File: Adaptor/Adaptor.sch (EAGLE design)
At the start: 10 parts

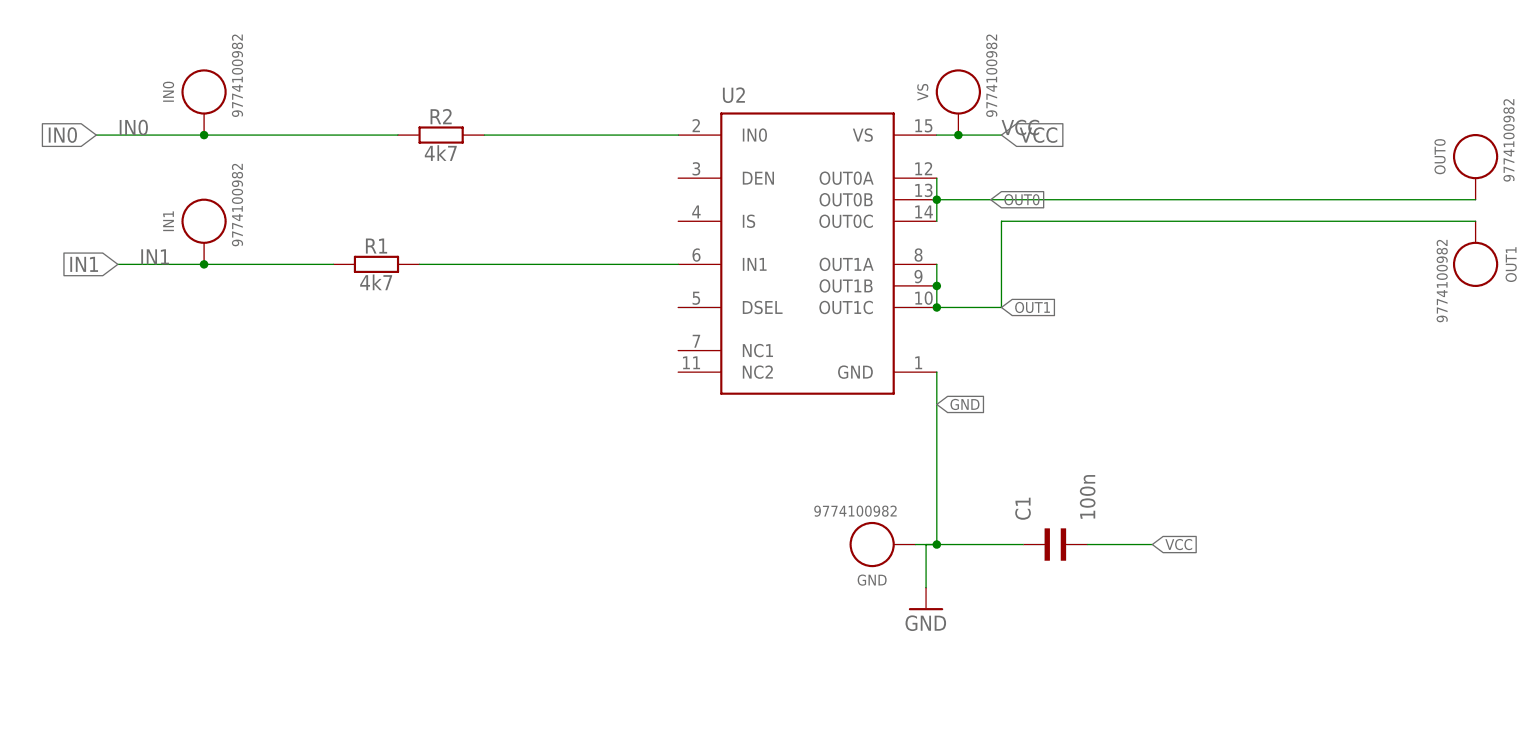
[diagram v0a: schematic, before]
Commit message: cleanm up.
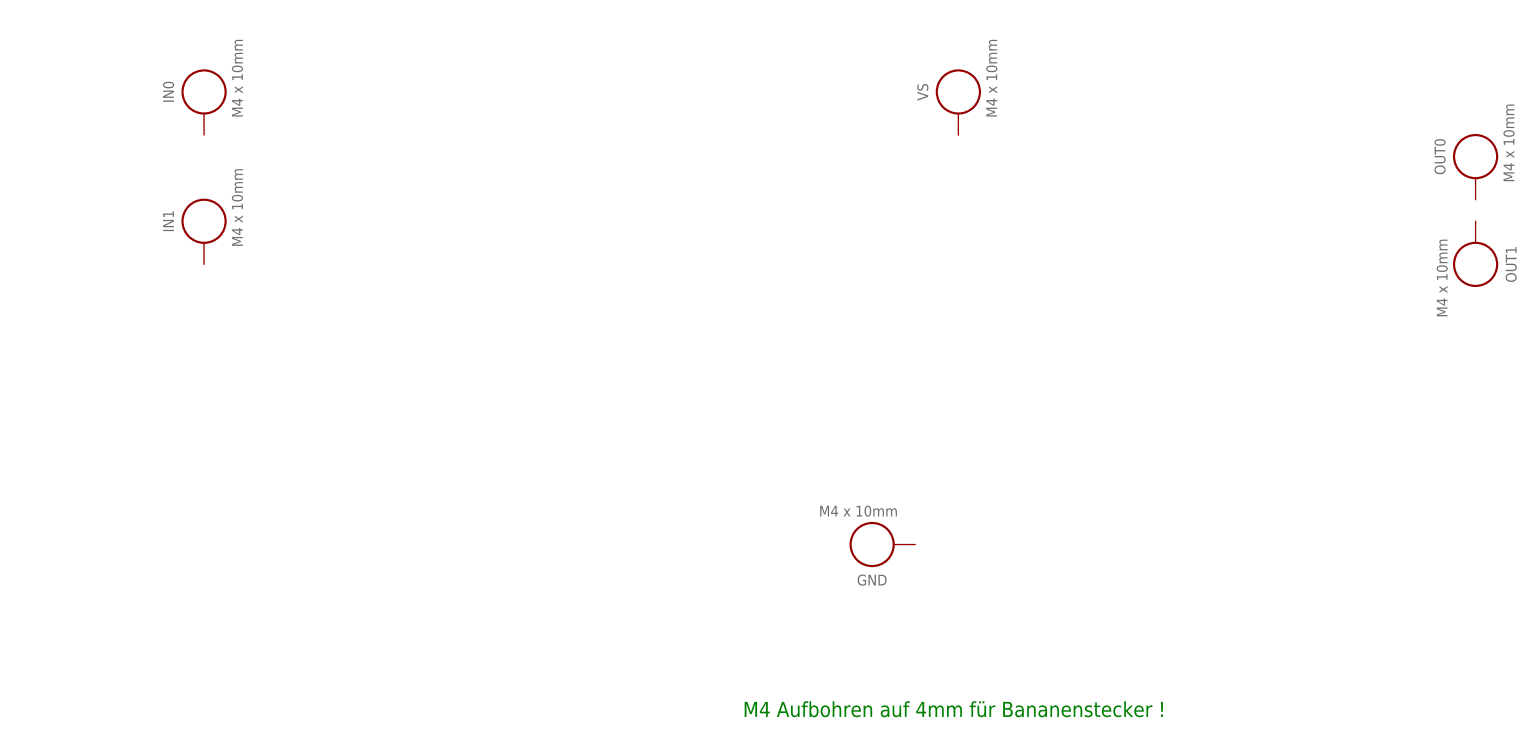
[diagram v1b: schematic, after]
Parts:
- removed C1: 100n, Wurth_Elektronik_Passive_Capacitors_rev19a:WCAP-CSGP_0402_885012205037
- removed R1, R2: 4k7, Resistor_smaller_fliegl:R-EU_WCAP-CSGP_0402
- removed U2: (no value), BTS7030-2EPA:BTS7030-2EPA
- GND, IN0, IN1, OUT0, OUT1, VS: value 9774100982 -> M4 x 10mm; device Wurth_Assembly_WA-SMST:WA-SMST_9774XXX982_9774100982 -> Wurth_Assembly_WA-SMSI:WA-SMSI_9774XXX482_9774100482
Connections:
- removed net GND: C1.2, GND.1, U2.GND
- removed net IN0: IN0.1, R2.1
- removed net IN1: IN1.1, R1.1
- removed net N$16: R2.2, U2.IN0
- removed net N$18: R1.2, U2.IN1
- removed net OUT0: OUT0.1, U2.OUT0A, U2.OUT0B, U2.OUT0C
- removed net OUT1: OUT1.1, U2.OUT1A, U2.OUT1B, U2.OUT1C
- removed net VCC: C1.1, U2.VS, VS.1
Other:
- note added: "M4 Aufbohren auf 4mm für Bananenstecker !"
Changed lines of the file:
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@@
 <drawing>
 <settings>
-<setting alwaysvectorfont="yes"/>
+<setting alwaysvectorfont="no"/>
 <setting verticaltext="up"/>
 </settings>
@@
 </classes>
 <parts>
-<part name="U2" library="BTS7030-2EPA" deviceset="BTS7030-2EPA" device=""/>
-<part name="R2" library="Resistor_smaller_fliegl" deviceset="R-EU_" device="WCAP-CSGP_0402" package3d_urn="urn:adsk.eagle:package:18563160/2" value="4k7"/>
-<part name="R1" library="Resistor_smaller_fliegl" deviceset="R-EU_" device="WCAP-CSGP_0402" package3d_urn="urn:adsk.eagle:package:18563160/2" value="4k7"/>
-<part name="GND21" library="supply1" library_urn="urn:adsk.eagle:library:371" deviceset="GND" device=""/>
-<part name="C1" library="Wurth_Elektronik_Passive_Capacitors_rev19a" library_urn="urn:adsk.eagle:library:491551" deviceset="WCAP-CSGP_0402" device="" package3d_urn="urn:adsk.eagle:package:491821/3" technology="_885012205037" value="100n"/>
-<part name="IN0" library="Wurth_Assembly_WA-SMST" library_urn="urn:adsk.eagle:library:14418621" deviceset="WA-SMST_9774XXX982" device="_9774100982" package3d_urn="urn:adsk.eagle:package:14328907/2" value=" 9774100982 "/>
-<part name="IN1" library="Wurth_Assembly_WA-SMST" library_urn="urn:adsk.eagle:library:14418621" deviceset="WA-SMST_9774XXX982" device="_9774100982" package3d_urn="urn:adsk.eagle:package:14328907/2" value=" 9774100982 "/>
-<part name="GND" library="Wurth_Assembly_WA-SMST" library_urn="urn:adsk.eagle:library:14418621" deviceset="WA-SMST_9774XXX982" device="_9774100982" package3d_urn="urn:adsk.eagle:package:14328907/2" value=" 9774100982 "/>
-<part name="OUT1" library="Wurth_Assembly_WA-SMST" library_urn="urn:adsk.eagle:library:14418621" deviceset="WA-SMST_9774XXX982" device="_9774100982" package3d_urn="urn:adsk.eagle:package:14328907/2" value=" 9774100982 "/>
-<part name="OUT0" library="Wurth_Assembly_WA-SMST" library_urn="urn:adsk.eagle:library:14418621" deviceset="WA-SMST_9774XXX982" device="_9774100982" package3d_urn="urn:adsk.eagle:package:14328907/2" value=" 9774100982 "/>
-<part name="VS" library="Wurth_Assembly_WA-SMST" library_urn="urn:adsk.eagle:library:14418621" deviceset="WA-SMST_9774XXX982" device="_9774100982" package3d_urn="urn:adsk.eagle:package:14328907/2" value=" 9774100982 "/>
+<part name="IN0" library="Wurth_Assembly_WA-SMSI" library_urn="urn:adsk.eagle:library:14418591" deviceset="WA-SMSI_9774XXX482" device="_9774100482" package3d_urn="urn:adsk.eagle:package:14321898/2" value="M4 x 10mm"/>
+<part name="IN1" library="Wurth_Assembly_WA-SMSI" library_urn="urn:adsk.eagle:library:14418591" deviceset="WA-SMSI_9774XXX482" device="_9774100482" package3d_urn="urn:adsk.eagle:package:14321898/2" value="M4 x 10mm"/>
+<part name="GND" library="Wurth_Assembly_WA-SMSI" library_urn="urn:adsk.eagle:library:14418591" deviceset="WA-SMSI_9774XXX482" device="_9774100482" package3d_urn="urn:adsk.eagle:package:14321898/2" value="M4 x 10mm"/>
+<part name="OUT1" library="Wurth_Assembly_WA-SMSI" library_urn="urn:adsk.eagle:library:14418591" deviceset="WA-SMSI_9774XXX482" device="_9774100482" package3d_urn="urn:adsk.eagle:package:14321898/2" value="M4 x 10mm"/>
+<part name="OUT0" library="Wurth_Assembly_WA-SMSI" library_urn="urn:adsk.eagle:library:14418591" deviceset="WA-SMSI_9774XXX482" device="_9774100482" package3d_urn="urn:adsk.eagle:package:14321898/2" value="M4 x 10mm"/>
+<part name="VS" library="Wurth_Assembly_WA-SMSI" library_urn="urn:adsk.eagle:library:14418591" deviceset="WA-SMSI_9774XXX482" device="_9774100482" package3d_urn="urn:adsk.eagle:package:14321898/2" value="M4 x 10mm"/>
 </parts>
 <sheets>
 <sheet>
 <plain>
+<text x="86.36" y="5.08" size="1.778" layer="91">M4 Aufbohren auf 4mm für Bananenstecker !</text>
 </plain>
 <instances>
-<instance part="U2" gate="G$1" x="83.82" y="76.2" smashed="yes">
-<attribute name="NAME" x="83.82" y="77.47" size="1.778" layer="95"/>
-<attribute name="VALUE" x="83.82" y="40.005" size="1.778" layer="96"/>
-</instance>
-<instance part="R2" gate="G$1" x="50.8" y="73.66" smashed="yes">
-<attribute name="NAME" x="50.8" y="74.93" size="1.778" layer="95" align="bottom-center"/>
-<attribute name="VALUE" x="50.8" y="72.39" size="1.778" layer="96" align="top-center"/>
-</instance>
-<instance part="R1" gate="G$1" x="43.18" y="58.42" smashed="yes">
-<attribute name="NAME" x="43.18" y="59.69" size="1.778" layer="95" align="bottom-center"/>
-<attribute name="VALUE" x="43.18" y="57.15" size="1.778" layer="96" align="top-center"/>
-</instance>
-<instance part="GND21" gate="1" x="107.95" y="17.78" smashed="yes">
-<attribute name="VALUE" x="105.41" y="15.24" size="1.778" layer="96"/>
-</instance>
-<instance part="C1" gate="G$1" x="124.46" y="25.4" smashed="yes" rot="R90">
-<attribute name="NAME" x="120.269" y="28.194" size="1.778" layer="95" rot="R90"/>
-<attribute name="VALUE" x="127.889" y="28.194" size="1.778" layer="96" rot="R90"/>
-</instance>
 <instance part="IN0" gate="G$1" x="22.86" y="78.74" smashed="yes" rot="R90">
 <attribute name="NAME" x="19.304" y="78.74" size="1.27" layer="95" rot="R90" align="bottom-center"/>
@@
 </busses>
 <nets>
-<net name="GND" class="0">
-<segment>
-<pinref part="GND21" gate="1" pin="GND"/>
-<wire x1="107.95" y1="25.4" x2="107.95" y2="20.32" width="0.1524" layer="91"/>
-<wire x1="107.95" y1="25.4" x2="109.22" y2="25.4" width="0.1524" layer="91"/>
-<pinref part="C1" gate="G$1" pin="2"/>
-<pinref part="U2" gate="G$1" pin="GND"/>
-<label x="109.22" y="41.91" size="1.27" layer="95" xref="yes"/>
-<wire x1="109.22" y1="25.4" x2="119.38" y2="25.4" width="0.1524" layer="91"/>
-<wire x1="109.22" y1="25.4" x2="109.22" y2="45.72" width="0.1524" layer="91"/>
-<junction x="109.22" y="25.4"/>
-<pinref part="GND" gate="G$1" pin="1"/>
-<wire x1="106.68" y1="25.4" x2="109.22" y2="25.4" width="0.1524" layer="91"/>
-</segment>
-</net>
-<net name="VCC" class="0">
-<segment>
-<pinref part="U2" gate="G$1" pin="VS"/>
-<wire x1="109.22" y1="73.66" x2="111.76" y2="73.66" width="0.1524" layer="91"/>
-<label x="116.84" y="73.66" size="1.778" layer="95"/>
-<label x="116.84" y="73.66" size="1.778" layer="95" xref="yes"/>
-<pinref part="VS" gate="G$1" pin="1"/>
-<wire x1="111.76" y1="73.66" x2="116.84" y2="73.66" width="0.1524" layer="91"/>
-<junction x="111.76" y="73.66"/>
-</segment>
-<segment>
-<pinref part="C1" gate="G$1" pin="1"/>
-<wire x1="127" y1="25.4" x2="134.62" y2="25.4" width="0.1524" layer="91"/>
-<label x="134.62" y="25.4" size="1.27" layer="95" xref="yes"/>
-</segment>
-</net>
-<net name="OUT0" class="0">
-<segment>
-<pinref part="U2" gate="G$1" pin="OUT0B"/>
-<pinref part="U2" gate="G$1" pin="OUT0A"/>
-<wire x1="172.72" y1="66.04" x2="109.22" y2="66.04" width="0.1524" layer="91"/>
-<wire x1="109.22" y1="68.58" x2="109.22" y2="66.04" width="0.1524" layer="91"/>
-<junction x="109.22" y="66.04"/>
-<pinref part="U2" gate="G$1" pin="OUT0C"/>
-<wire x1="109.22" y1="63.5" x2="109.22" y2="66.04" width="0.1524" layer="91"/>
-<label x="115.57" y="66.04" size="1.27" layer="95" xref="yes"/>
-<pinref part="OUT0" gate="G$1" pin="1"/>
-</segment>
-</net>
-<net name="OUT1" class="0">
-<segment>
-<pinref part="U2" gate="G$1" pin="OUT1C"/>
-<wire x1="172.72" y1="63.5" x2="116.84" y2="63.5" width="0.1524" layer="91"/>
-<wire x1="116.84" y1="63.5" x2="116.84" y2="53.34" width="0.1524" layer="91"/>
-<wire x1="116.84" y1="53.34" x2="109.22" y2="53.34" width="0.1524" layer="91"/>
-<pinref part="U2" gate="G$1" pin="OUT1B"/>
-<pinref part="U2" gate="G$1" pin="OUT1A"/>
-<wire x1="109.22" y1="55.88" x2="109.22" y2="58.42" width="0.1524" layer="91"/>
-<wire x1="109.22" y1="53.34" x2="109.22" y2="55.88" width="0.1524" layer="91"/>
-<junction x="109.22" y="53.34"/>
-<junction x="109.22" y="55.88"/>
-<label x="116.84" y="53.34" size="1.27" layer="95" xref="yes"/>
-<pinref part="OUT1" gate="G$1" pin="1"/>
-</segment>
-</net>
-<net name="IN1" class="0">
-<segment>
-<label x="15.24" y="58.42" size="1.778" layer="95"/>
-<label x="12.7" y="58.42" size="1.778" layer="95" rot="R180" xref="yes"/>
-<wire x1="38.1" y1="58.42" x2="22.86" y2="58.42" width="0.1524" layer="91"/>
-<pinref part="R1" gate="G$1" pin="1"/>
-<pinref part="IN1" gate="G$1" pin="1"/>
-<wire x1="22.86" y1="58.42" x2="12.7" y2="58.42" width="0.1524" layer="91"/>
-<junction x="22.86" y="58.42"/>
-</segment>
-</net>
-<net name="IN0" class="0">
-<segment>
-<label x="12.7" y="73.66" size="1.778" layer="95"/>
-<label x="10.16" y="73.66" size="1.778" layer="95" rot="R180" xref="yes"/>
-<wire x1="45.72" y1="73.66" x2="22.86" y2="73.66" width="0.1524" layer="91"/>
-<pinref part="R2" gate="G$1" pin="1"/>
-<pinref part="IN0" gate="G$1" pin="1"/>
-<wire x1="22.86" y1="73.66" x2="10.16" y2="73.66" width="0.1524" layer="91"/>
-<junction x="22.86" y="73.66"/>
-</segment>
-</net>
-<net name="N$16" class="0">
-<segment>
-<pinref part="U2" gate="G$1" pin="IN0"/>
-<pinref part="R2" gate="G$1" pin="2"/>
-<wire x1="55.88" y1="73.66" x2="78.74" y2="73.66" width="0.1524" layer="91"/>
-</segment>
-</net>
-<net name="N$18" class="0">
-<segment>
-<pinref part="U2" gate="G$1" pin="IN1"/>
-<pinref part="R1" gate="G$1" pin="2"/>
-<wire x1="48.26" y1="58.42" x2="78.74" y2="58.42" width="0.1524" layer="91"/>
-</segment>
-</net>
 </nets>
 </sheet>
